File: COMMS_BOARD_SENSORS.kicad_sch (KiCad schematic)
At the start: 27 parts, among them IC2 BMM350, J4 Screw_Terminal_01x02, J6 Conn_Coaxial_Small, U1 MAX31855KASA, U4 MAX-M10S, U6 MS5611-01BA

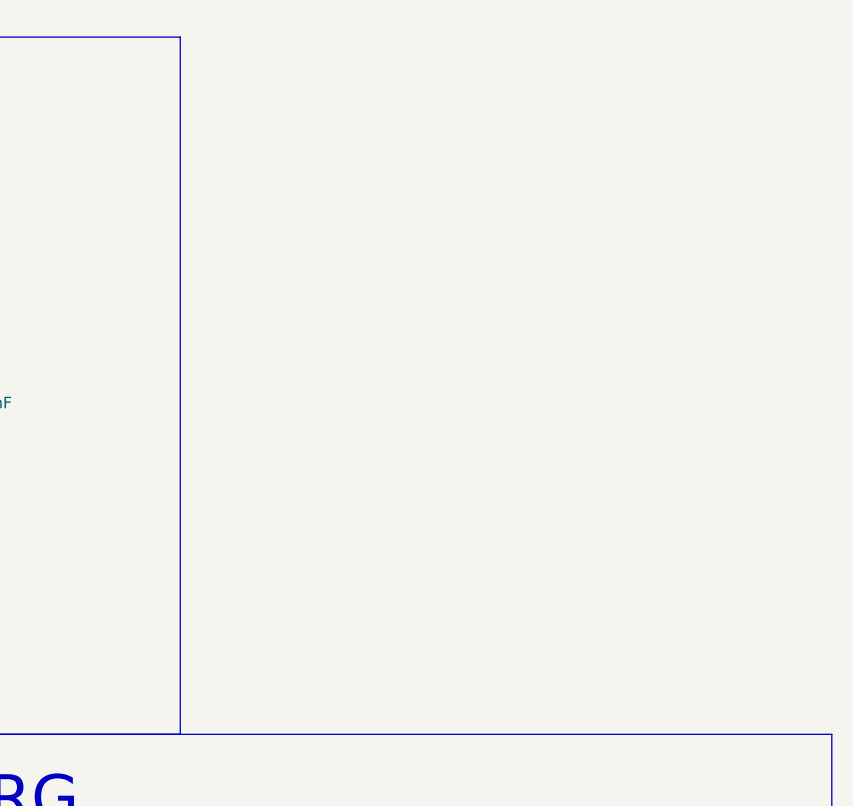
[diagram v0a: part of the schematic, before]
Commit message: ADDE IMU
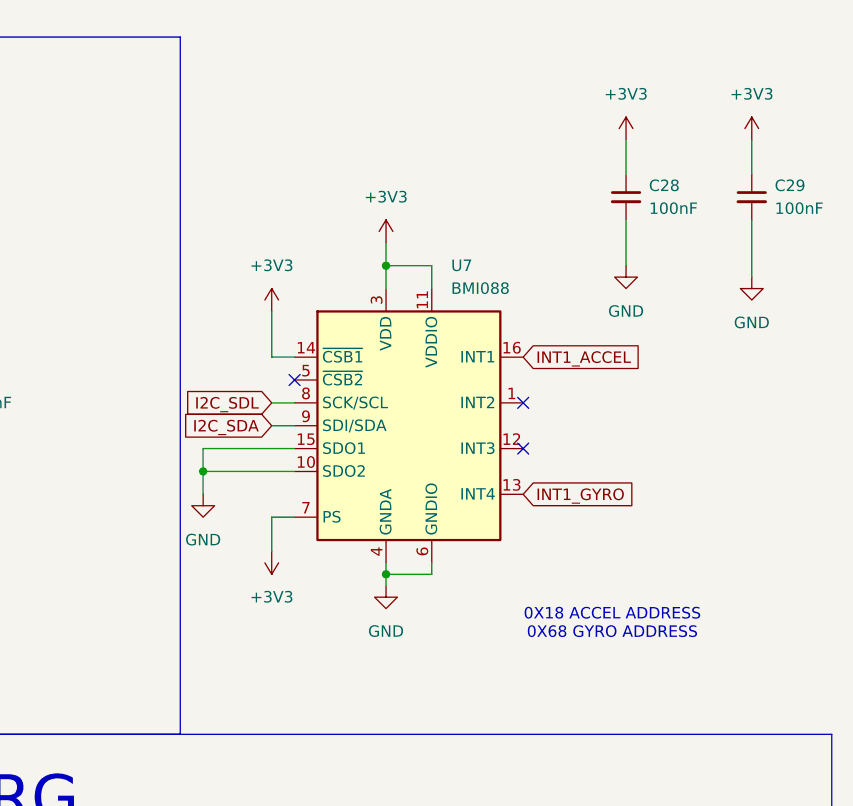
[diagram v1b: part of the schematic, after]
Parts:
- added C28, C29: 100nF, Capacitor_SMD:C_0603_1608Metric, symbol Device:C_Small
- added U7: BMI088, Package_LGA:Bosch_LGA-16_4.5x3mm_P0.5mm_LayoutBorder7x1y_ClockwisePinNumbering, symbol Sensor_Motion:BMI088
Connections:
- net +3V3: now also C28.1, C29.1, U7.11 (VDDIO), U7.14 (~{CSB1}), U7.3 (VDD), U7.7 (PS)
- net GND: now also C28.2, C29.2, U7.10 (SDO2), U7.15 (SDO1), U7.2 (GNDA), U7.4 (GNDA), U7.6 (GNDIO)
- net I2C_SDA: now also U7.9 (SDI/SDA)
- net I2C_SDL: now also U7.8 (SCK/SCL)
- new net INT1_ACCEL: U7.16 (INT1)
- new net INT1_GYRO: U7.13 (INT4)
- no-connect marks 10 -> 13
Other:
- note added: "0X18 ACCEL ADDRESS 0X68 GYRO ADDRESS"
